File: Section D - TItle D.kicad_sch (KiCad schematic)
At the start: 6 parts, among them J1 Conn_01x02_Pin, J2 Conn_01x02_Pin, J3 Conn_01x02_Pin, J4 Conn_01x02_Pin, J5 Conn_01x04_Socket, J6 Conn_01x05_Pin

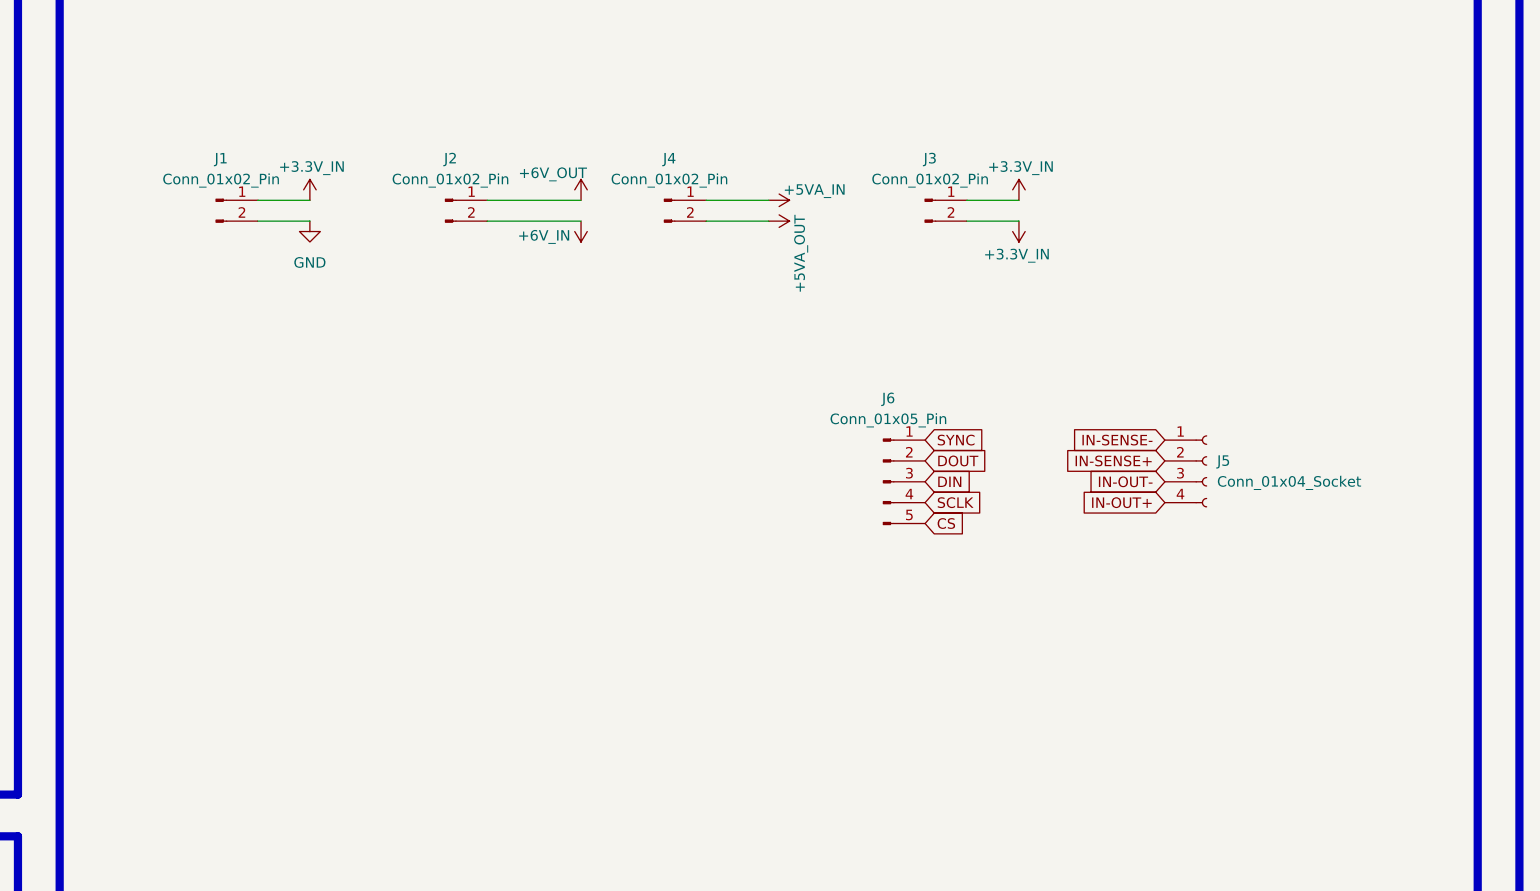
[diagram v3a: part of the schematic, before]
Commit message: [PCB 4 layer]
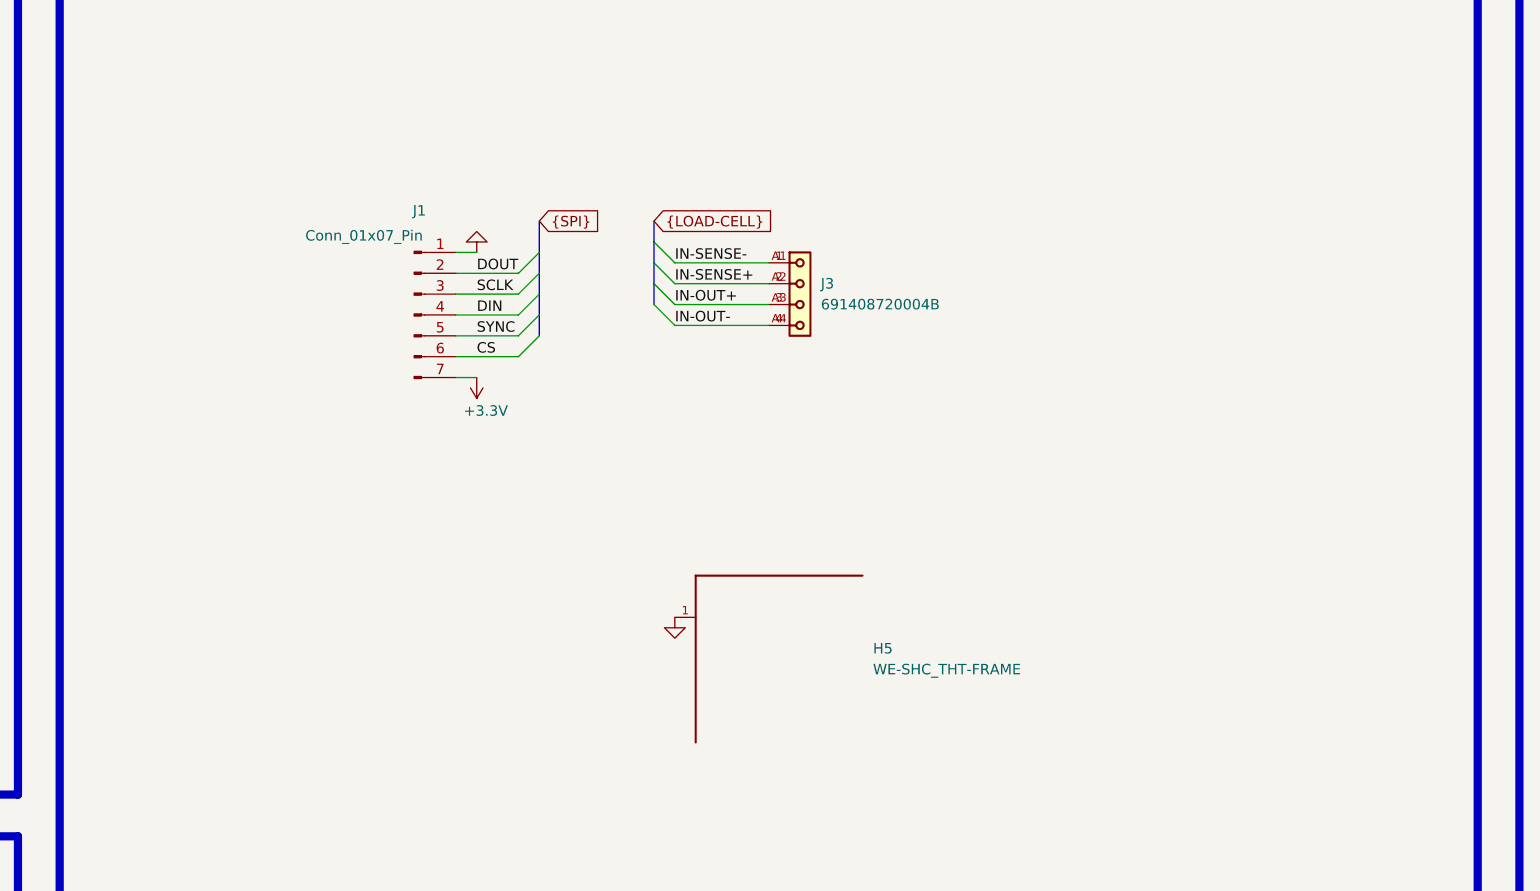
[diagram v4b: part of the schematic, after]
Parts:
- removed J1, J2, J3, J4: Conn_01x02_Pin, Connector_PinHeader_2.54mm:PinHeader_1x02_P2.54mm_Vertical, symbol Connector:Conn_01x02_Pin
- removed J5: Conn_01x04_Socket, Connector_PinSocket_2.54mm:PinSocket_1x04_P2.54mm_Vertical, symbol Connector:Conn_01x04_Socket
- removed J6: Conn_01x05_Pin, Connector_PinSocket_2.54mm:PinSocket_1x05_P2.54mm_Vertical, symbol Connector:Conn_01x05_Pin
- added H5: WE-SHC_THT-FRAME, WE-SHC_THT-FRAME:WE-SHC_THT-FRAME_36503205, symbol WE-SHC_THT-FRAME:WE-SHC_THT-FRAME
- added J1: Conn_01x07_Pin, Connector_JST:JST_XH_B7B-XH-AM_1x07_P2.50mm_Vertical, symbol Connector:Conn_01x07_Pin
- added J3: 691408720004B, 691408720004B:691408720004B, symbol 691408720004B:691408720004B
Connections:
- net CS: now also J1.6 (Pin_6)
- net DIN: now also J1.4 (Pin_4)
- net DOUT: now also J1.2 (Pin_2)
- net GND: now also H5.1, H5.10, H5.11, H5.12, H5.13, H5.14, H5.15, H5.16, H5.17, H5.2, H5.3, H5.4, H5.5, H5.6, H5.7, H5.9, J1.1 (Pin_1)
- net IN-OUT+: now also J3.3, J3.A3
- net IN-OUT-: now also J3.4, J3.A4
- net IN-SENSE+: now also J3.2, J3.A2
- net IN-SENSE-: now also J3.1, J3.A1
- net SCLK: now also J1.3 (Pin_3)
- net SYNC: now also J1.5 (Pin_5)
- new net +3.3V: J1.7 (Pin_7)
